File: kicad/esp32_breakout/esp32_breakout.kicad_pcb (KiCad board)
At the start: 2 copper layers, 78 x 39 mm, 30 parts, among them J1 JST PH F, J10 JST PH F, J11 JST PH F, J2 JST PH F, J3 JST PH F, J4 DC-005 5.5x2.1mm, J5 Deans T-Plug M, J6 Header F, J7 Header F, J8 Header F, J9 JST PH F, Q1 BSS123, SW1 SS12D10, U1 ESP32 DEV KIT 30-pin, U2 Mini560-Pro

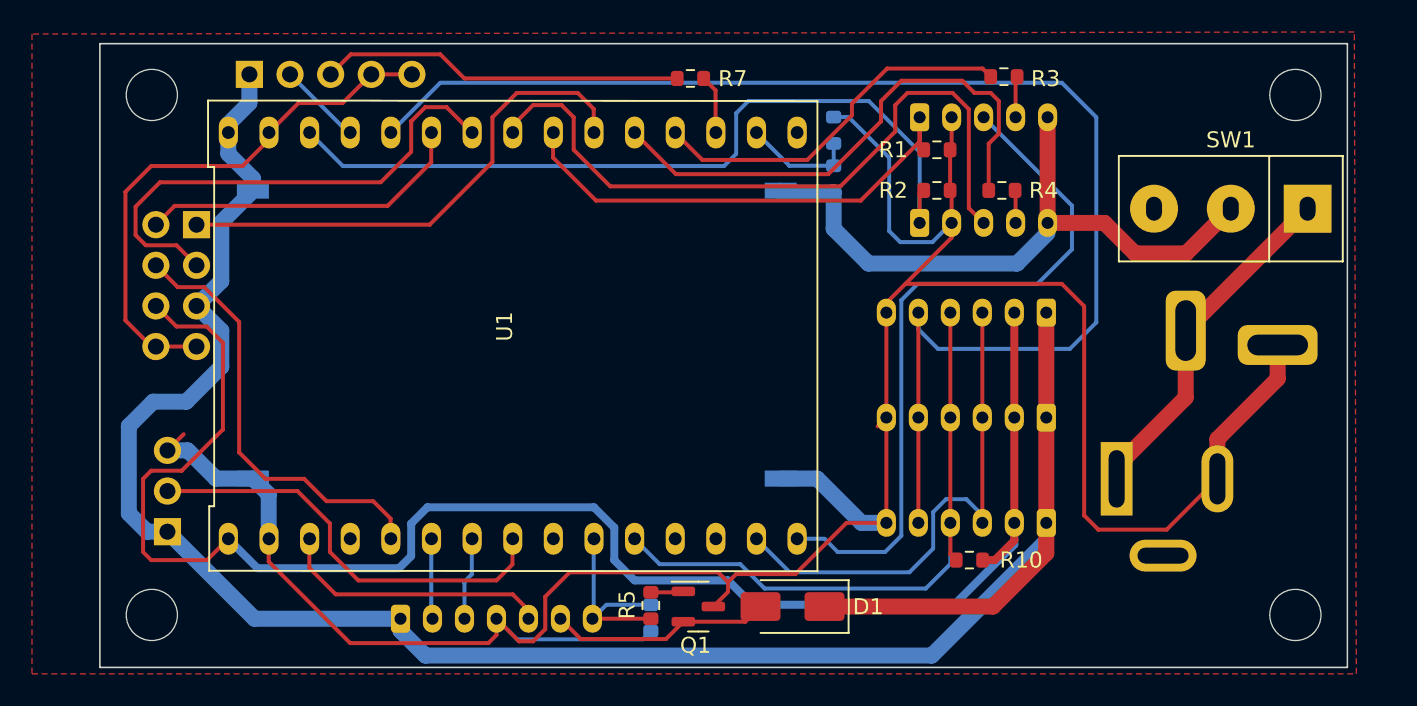
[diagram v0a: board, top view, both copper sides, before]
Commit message: PCB updated to product
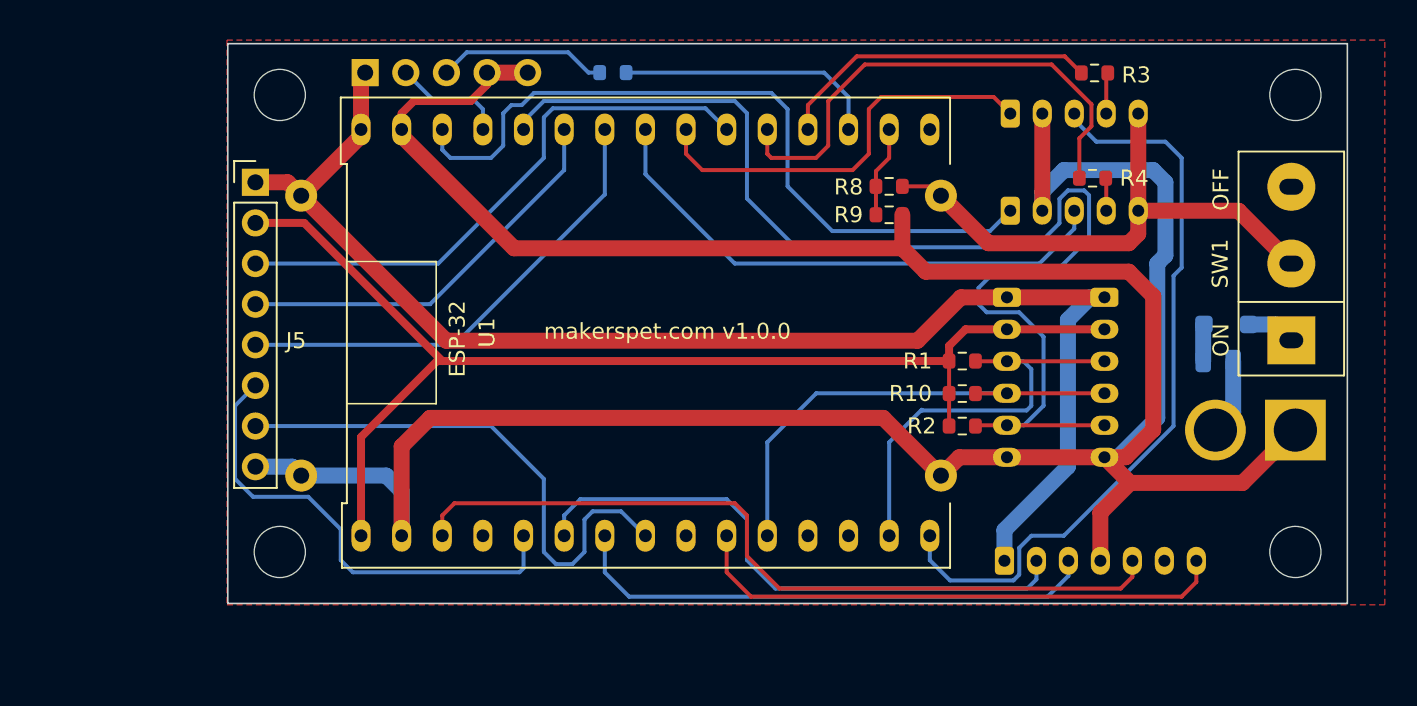
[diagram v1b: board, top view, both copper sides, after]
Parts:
- removed D1: CGRA4004-G, Diode_SMD:D_SMA
- removed J11: JST PH F, Connector_JST:JST_PH_B6B-PH-K_1x06_P2.00mm_Vertical
- removed the J6 at (123.6, 89.5)
- removed J8: Header F, Connector_PinHeader_2.54mm:PinHeader_1x03_P2.54mm_Vertical
- removed Q1: BSS123, Package_TO_SOT_SMD:SOT-23
- removed R5: 1k, Resistor_SMD:R_0603_1608Metric
- removed R6: 10k, Resistor_SMD:R_0603_1608Metric
- added D2: FS26, Diode_SMD:D_SOD-123F, B.Cu at (188.0, 95.8)
- added F1: FCC20202AATP, Fuse:Fuse_0805_2012Metric, B.Cu at (187.5, 98.0)
- J4: value DC-005 5.5x2.1mm -> XT30U-M; footprint Connector_BarrelJack:BarrelJack_GCT_DCJ200-10-A_Horizontal -> Connector_AMASS:AMASS_XT30U-M_1x02_P5.0mm_Vertical
- J5: value Deans T-Plug M -> J5; footprint Makerspet:DEANS-T-PLUG -> Connector_PinHeader_2.54mm:PinHeader_1x08_P2.54mm_Vertical; moved to F.Cu
- J6: renamed from J7; value Header F -> Header F 2.54mm
- R10: value 4.7k -> 10k
- R7: moved to B.Cu
- R8: moved to F.Cu
- R9: value 100k -> 10k; moved to F.Cu
- U2: value Mini560-Pro -> U2; footprint Makerspet:Mini560-Pro -> Makerspet:LM2596 Module
- moved J5 61.8 mm to (127.3, 86.9), turned to 0 degrees
- moved J3 37.9 mm to (174.1, 110.5)
- moved R2 14.8 mm to (171.4, 102.1)
- moved R1 13.3 mm to (171.4, 98.0)
- moved J4 11.6 mm to (192.3, 102.4), turned to 180 degrees
- moved R10 10.4 mm to (171.4, 100.1), turned to 0 degrees
- moved H4 8.92 mm to (128.8, 110.0)
- moved J10 8.35 mm to (180.3, 94.1), turned to -90 degrees
- moved U1 8.30 mm to (151.6, 96.3)
- moved H1 8.00 mm to (128.8, 81.4)
- moved J6 7.24 mm to (134.1, 80.0)
- moved U2 6.52 mm to (150.1, 96.5)
- moved R9 6.32 mm to (166.9, 88.9), turned to 180 degrees
- moved J1 5.72 mm to (174.5, 88.6)
- moved R4 5.72 mm to (179.6, 86.6)
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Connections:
- J3 pad 6: Net-(D1-A) -> unconnected-(J3-Pin_6-Pad6)
- J4 pad 1: +BATT -> GND
- J4 pad 2: GND -> Net-(J4-+)
- J5 pad 1: +BATT -> +5V
- J5 pad 2: GND -> +3V3
- R1 pad 1: /MOT_PWM_LEFT -> +3V3
- R1 pad 2: GND -> /I2C_SCL
- R2 pad 1: /MOT_PWM_RIGHT -> +3V3
- R2 pad 2: GND -> /I2C_INT
- SW1 pad 1: +BATT -> Net-(D2-K)
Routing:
- net +5V: track 129.3 -> 87.2 mm
- net /LDS_MOT_PWM: track 17.2 -> 49.7 mm
- net /LDS_TX: track 5.03 -> 36.4 mm
- net +3V3: track 103.6 -> 75.3 mm
- net /LDS_RX: track 5.22 -> 33.4 mm
- net +BATT: track 21.8 -> 0.00 mm
- net /LDS_MOT_EN: track 12.7 -> 34.0 mm
- net Net-(D1-A): track 13.9 -> 0.00 mm
- net /GPIO39_IN: track 3.69 -> 16.6 mm
- net Net-(J6-Pin_3): track 22.8 -> 10.6 mm
- net /MOT_CW_RIGHT: track 44.1 -> 33.9 mm
- net /I2C_SDA: track 39.9 -> 30.2 mm
- net /I2C_INT: track 85.9 -> 77.8 mm
- net /GPIO5_BOOT_STRAP: track 26.9 -> 33.8 mm
- net +24V: track 41.3 -> 34.9 mm
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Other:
- board size 78 x 39 mm -> 70 x 35 mm
- board text added: "BATT"
- board text added: "DIST"
- board text added: "EXT"
- board text added: "LEFT"
- board text added: "LM2596 DC-DC Module"
- board text added: "MOTORS"
- board text added: "OFF"
- board text added: "ON"
- board text added: "RIGHT"
- board text added: "makerspet.com v1.0.0"
